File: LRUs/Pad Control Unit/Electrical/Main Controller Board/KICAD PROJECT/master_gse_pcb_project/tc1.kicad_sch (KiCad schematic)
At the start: 21 parts, among them J18 B4B-XH-A, U26 MAX31856, U27 MAX31856

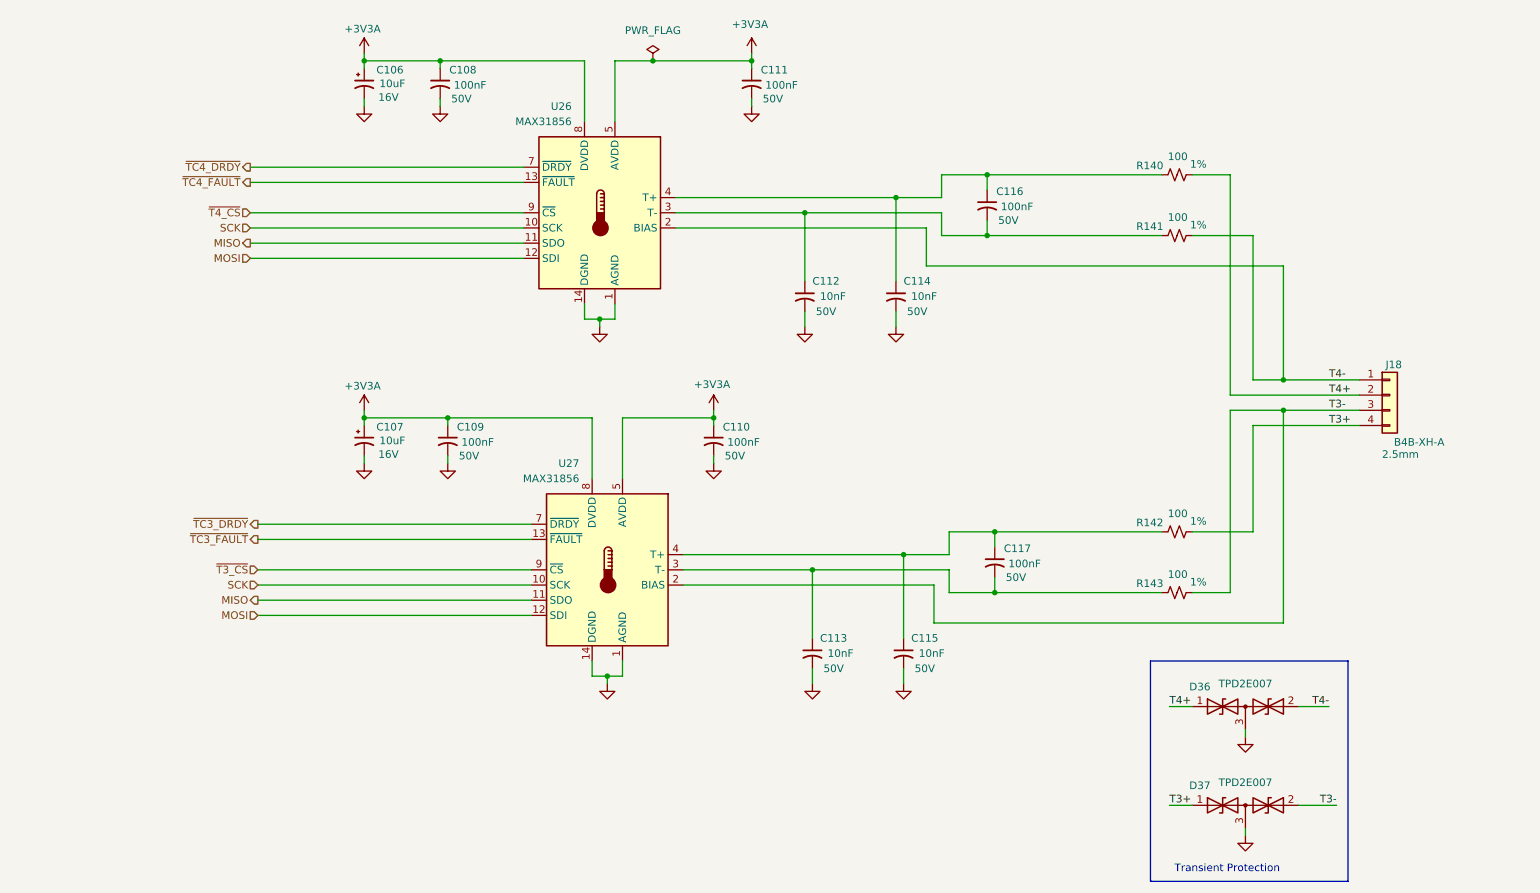
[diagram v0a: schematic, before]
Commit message: Committ latest changes
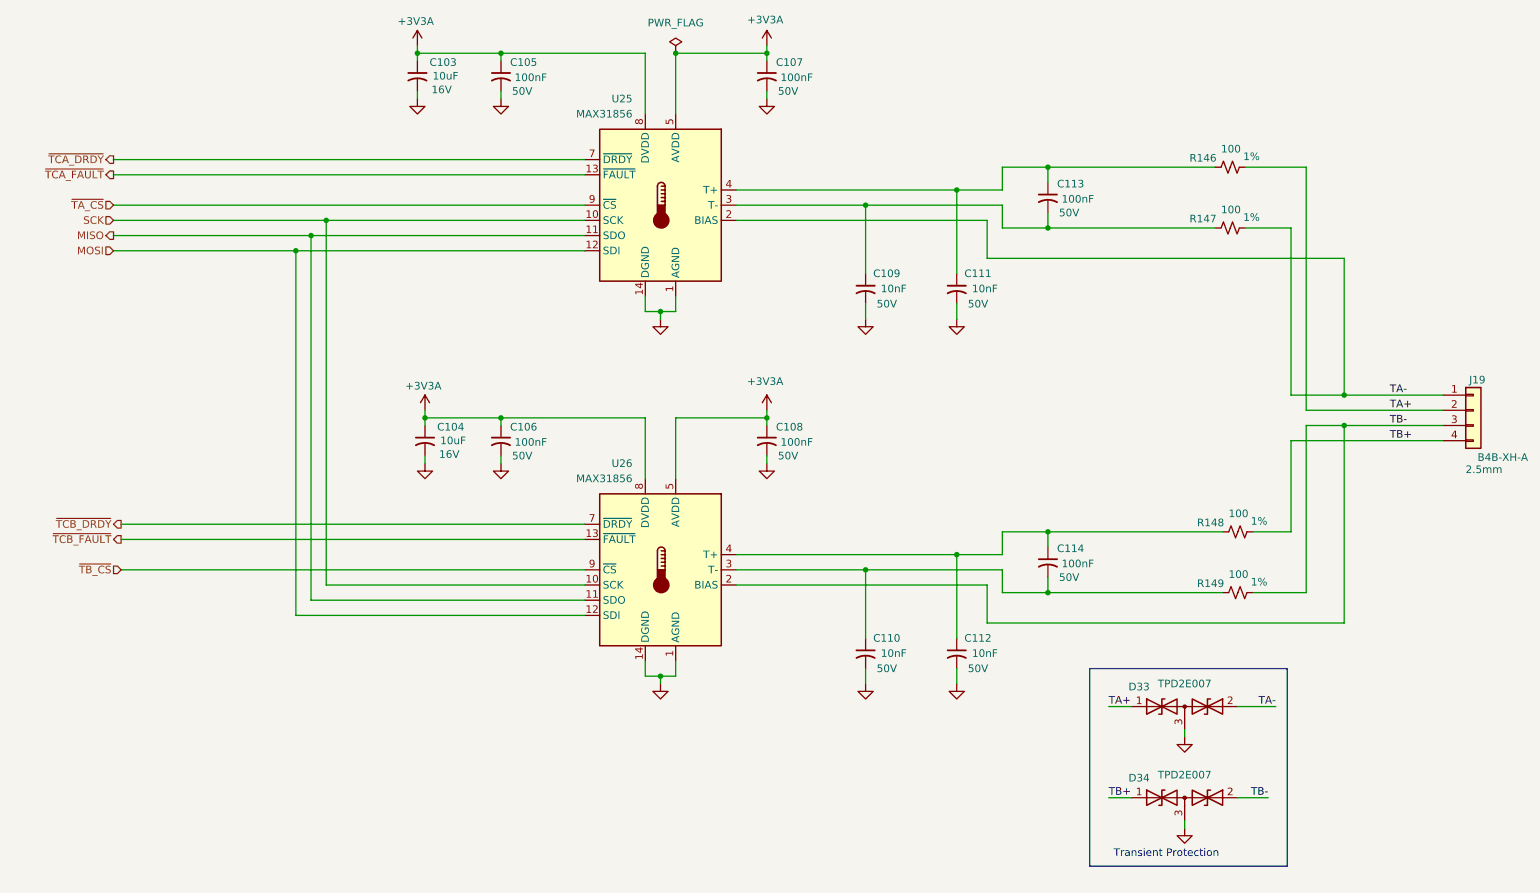
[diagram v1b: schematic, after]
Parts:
- removed C106, C107: 10uF, Capacitor_Tantalum_SMD:CP_EIA-3216-18_Kemet-A, symbol Device:C_Polarized_Small_US
- added C103, C104: 10uF, Capacitor_SMD:C_0805_2012Metric, symbol Device:C_Small_US
- renumbered C109 to C105, C108 to C106, C110 to C107, C111 to C108, C113 to C109, C112 to C110, C115 to C111, C114 to C112, C117 to C113, C116 to C114, D37 to D33, D36 to D34, J18 to J19, R142 to R146, R143 to R147, R140 to R148, R141 to R149, U27 to U25
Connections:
- net +3V3A: now also C103.1, C104.1
- net GND: now also C103.2, C104.2
- net T3+ renamed TA+
- net TA+: now also J19.2 (Pin_2); no longer J19.4 (Pin_4)
- net T3- renamed TA-
- net TA-: now also J19.1 (Pin_1); no longer J19.3 (Pin_3)
- net T4+ renamed TB+
- net TB+: now also J19.4 (Pin_4); no longer J19.2 (Pin_2)
- net T4- renamed TB-
- net TB-: now also J19.3 (Pin_3); no longer J19.1 (Pin_1)
- net ~{T3_CS} renamed ~{TA_CS}
- net ~{T4_CS} renamed ~{TB_CS}
- net ~{TC3_DRDY} renamed ~{TCA_DRDY}
- net ~{TC3_FAULT} renamed ~{TCA_FAULT}
- net ~{TC4_DRDY} renamed ~{TCB_DRDY}
- net ~{TC4_FAULT} renamed ~{TCB_FAULT}
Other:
- moved on the sheet: C105, C106, C107, C108, C109, C110, C111, C112, C113, C114, D33, D34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
